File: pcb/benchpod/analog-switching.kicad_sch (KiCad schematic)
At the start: 8 parts, among them U53 TPL7407LAPWR, U58 TCA9554PWR

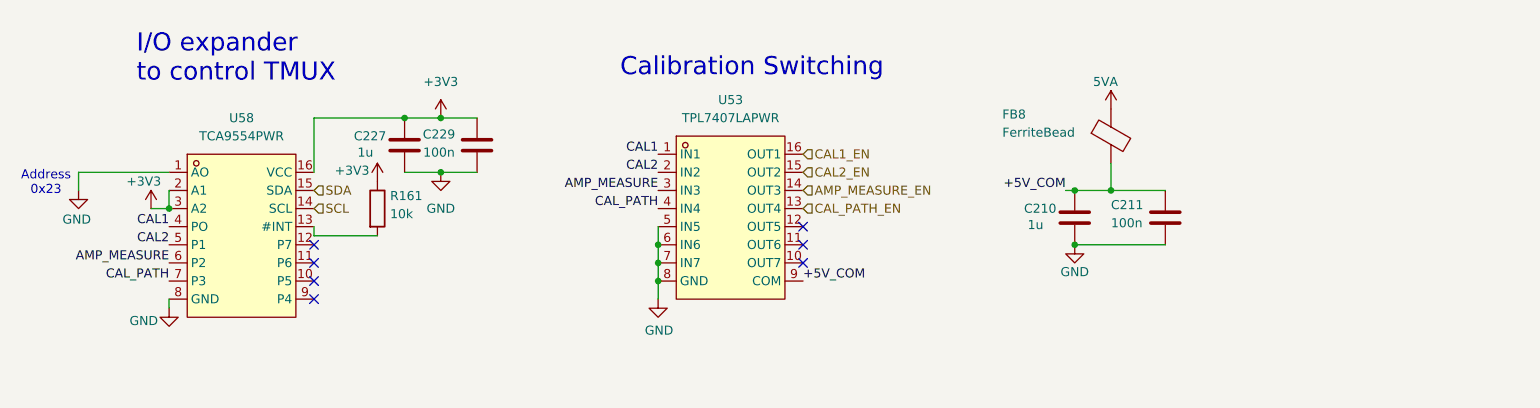
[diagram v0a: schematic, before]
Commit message: fix pull-downs for board boot-up
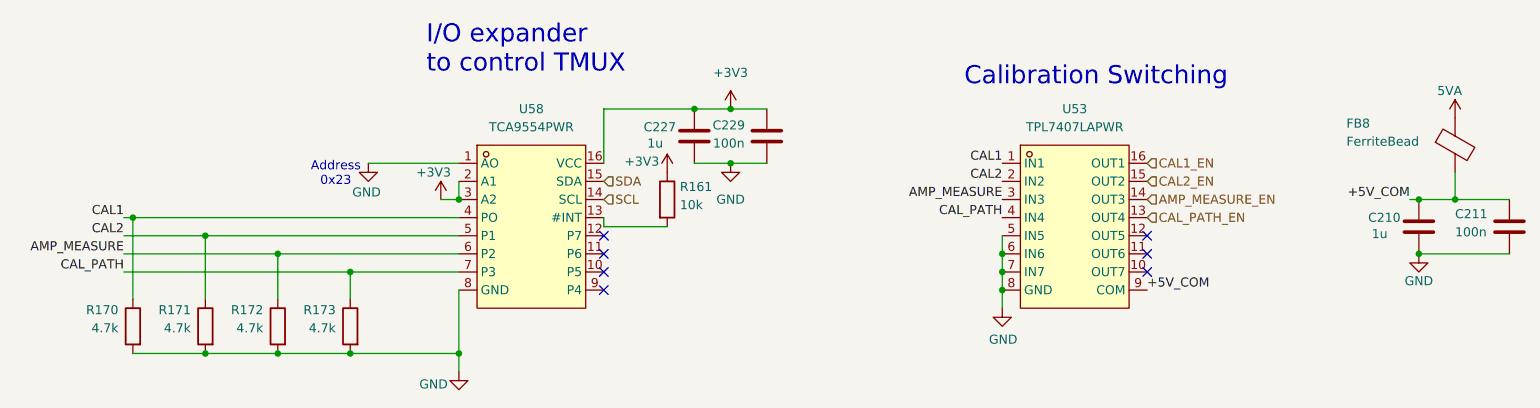
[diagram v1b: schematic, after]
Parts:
- added R170, R171, R172, R173: 4.7k, Resistor_SMD:R_0402_1005Metric, symbol Device:R
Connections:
- net AMP_MEASURE: now also R172.1
- net CAL1: now also R170.1
- net CAL2: now also R171.1
- net CAL_PATH: now also R173.1
- net GND: now also R170.2, R171.2, R172.2, R173.2
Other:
- moved on the sheet: C210, C211, C227, C229, FB8, R161, U53, U58
